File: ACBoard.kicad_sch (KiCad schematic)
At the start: 25 parts, among them J1 Conn_02x20_Odd_Even, J2 Conn_02x20_Odd_Even, J3 Conn_01x02_Male, J4 Conn_01x02_Female, J5 Conn_01x02_Female, T1 CSE185L, U1 TLP561, U2 TLP561, U3 ADS7822U

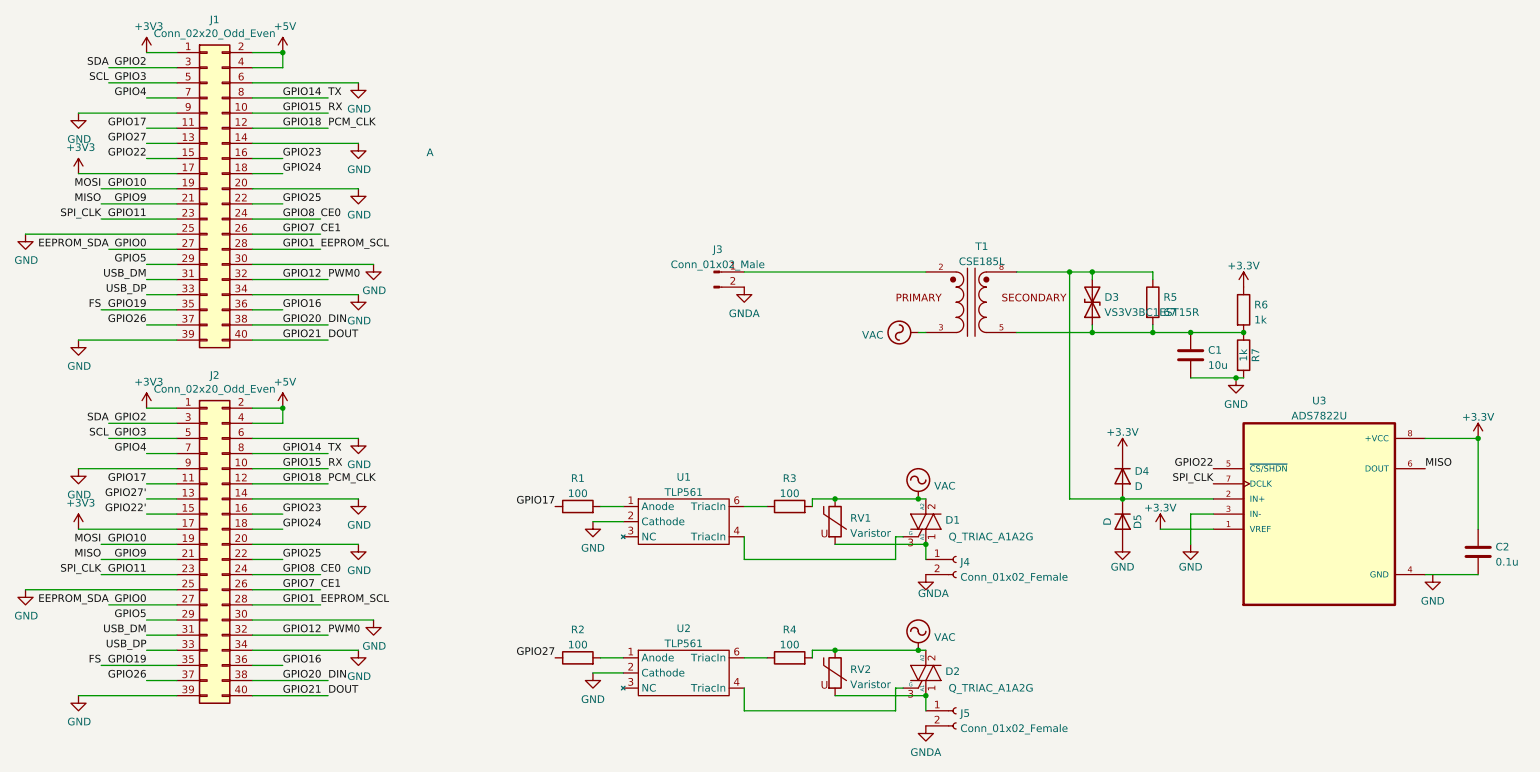
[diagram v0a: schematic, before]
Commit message: data5
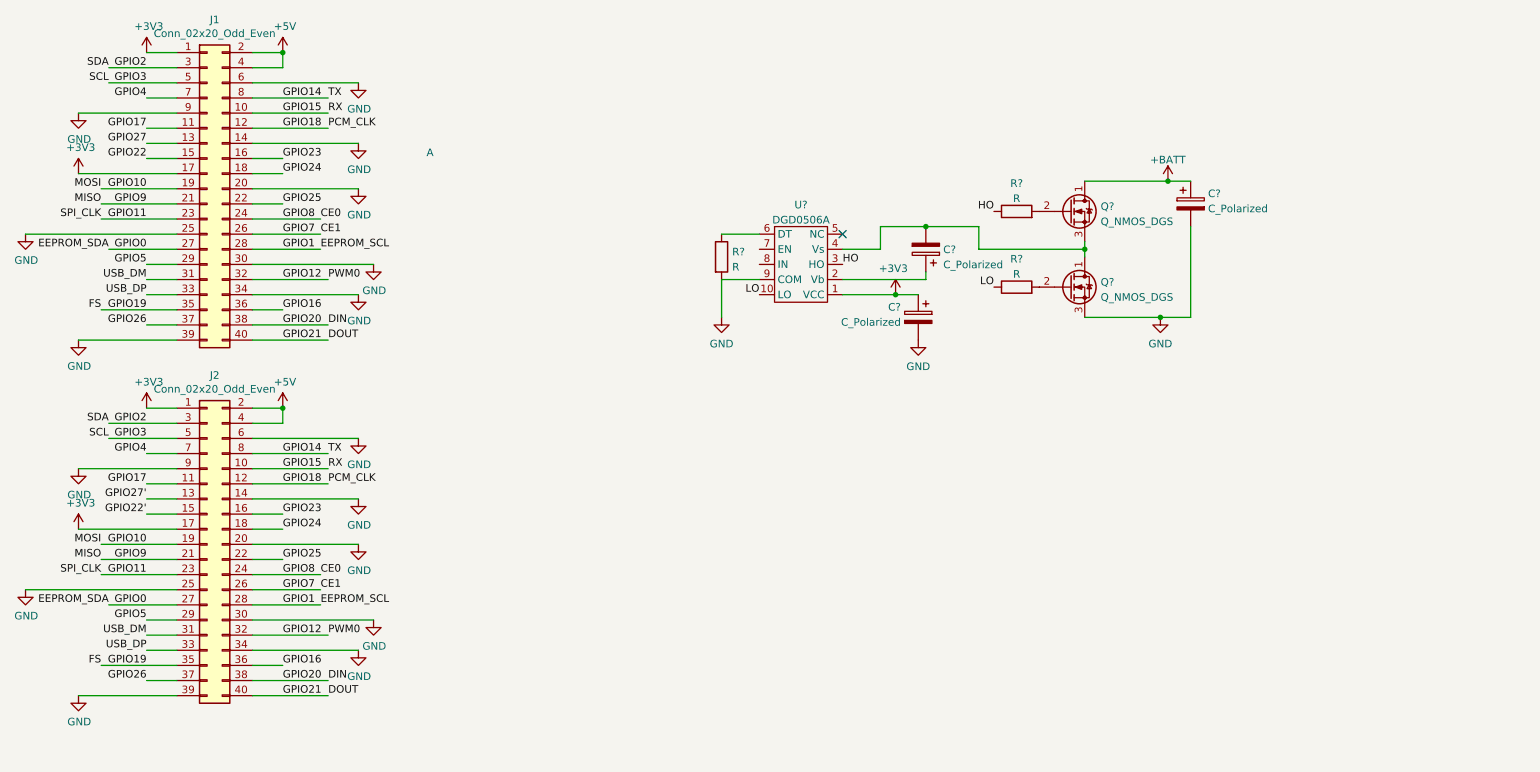
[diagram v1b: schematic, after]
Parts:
- removed C1: 10u, Capacitor_SMD:C_0805_2012Metric_Pad1.18x1.45mm_HandSolder, symbol Device:C
- removed C2: 0.1u, Capacitor_SMD:C_1206_3216Metric_Pad1.33x1.80mm_HandSolder, symbol Device:C
- removed D1, D2: Q_TRIAC_A1A2G, Package_TO_SOT_THT:TO-220-3_Horizontal_TabDown, symbol Device:Q_TRIAC_A1A2G
- removed D3: VS3V3BC1EST15R, Diode_SMD:D_0201_0603Metric_Pad0.64x0.40mm_HandSolder, symbol Device:D_TVS
- removed D4, D5: D, Diode_THT:D_5W_P12.70mm_Horizontal, symbol Device:D
- removed J3: Conn_01x02_Male, locallib:ACinlet, symbol Connector:Conn_01x02_Male
- removed J4, J5: Conn_01x02_Female, locallib:AcOutlet, symbol Connector:Conn_01x02_Female
- removed R1, R2, R3, R4: 100, Resistor_SMD:R_0603_1608Metric_Pad0.98x0.95mm_HandSolder, symbol Device:R
- removed R5: 67, Resistor_SMD:R_0603_1608Metric_Pad0.98x0.95mm_HandSolder, symbol Device:R
- removed R6, R7: 1k, Resistor_SMD:R_0603_1608Metric_Pad0.98x0.95mm_HandSolder, symbol Device:R
- removed RV1, RV2: Varistor, Varistor:RV_Disc_D9mm_W3.8mm_P5mm, symbol Device:Varistor
- removed T1: CSE185L, locallib:XFMR_CSE185L, symbol locallib:CSE185L
- removed U1, U2: TLP561, Package_DIP:DIP-5-6_W7.62mm, symbol locallib:TLP561
- removed U3: ADS7822U, locallib:SOIC127P599X175-8N, symbol locallib:ADS7822U
- added C? (x3): C_Polarized, symbol Device:C_Polarized
- added Q? (x2): Q_NMOS_DGS, symbol Device:Q_NMOS_DGS
- added R? (x3): R, symbol Device:R
- added U?: DGD0506A, symbol locallib:DGD0506A
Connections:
- net +3V3: now also C?.1, U?.1 (VCC)
- net GND: now also C?.2, C?.2, Q?.3 (S), R?.2, U?.9 (COM)
- new net: C?.1, U?.2 (Vb)
- new net: C?.2, Q?.1 (D), Q?.3 (S), U?.4 (Vs)
- new net: Q?.2 (G), R?.2 (x2)
- new net: R?.1, U?.6 (DT)
- new net +BATT: C?.1, Q?.1 (D)
- new net HO: R?.1, U?.3 (HO)
- new net LO: R?.1, U?.10 (LO)
- no-connect marks 0 -> 1
